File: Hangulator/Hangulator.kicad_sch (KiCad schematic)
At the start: 78 parts, among them J1 Conn_01x02_Male, J2 Conn_01x02_Male, U1 AMS1117-3.3, U2 STM32F072VBTx

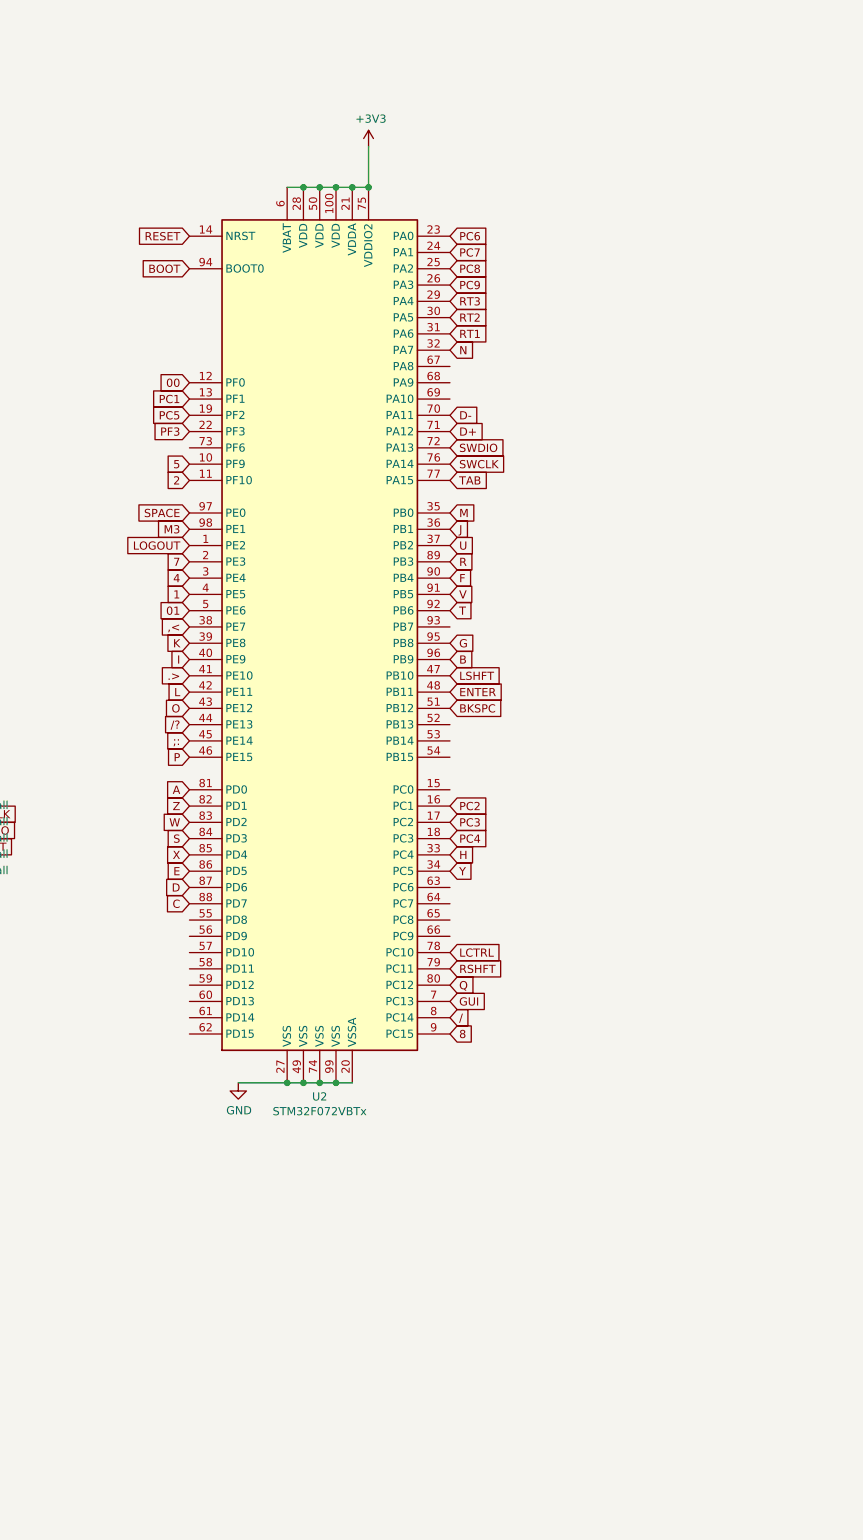
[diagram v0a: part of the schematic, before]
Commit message: lol
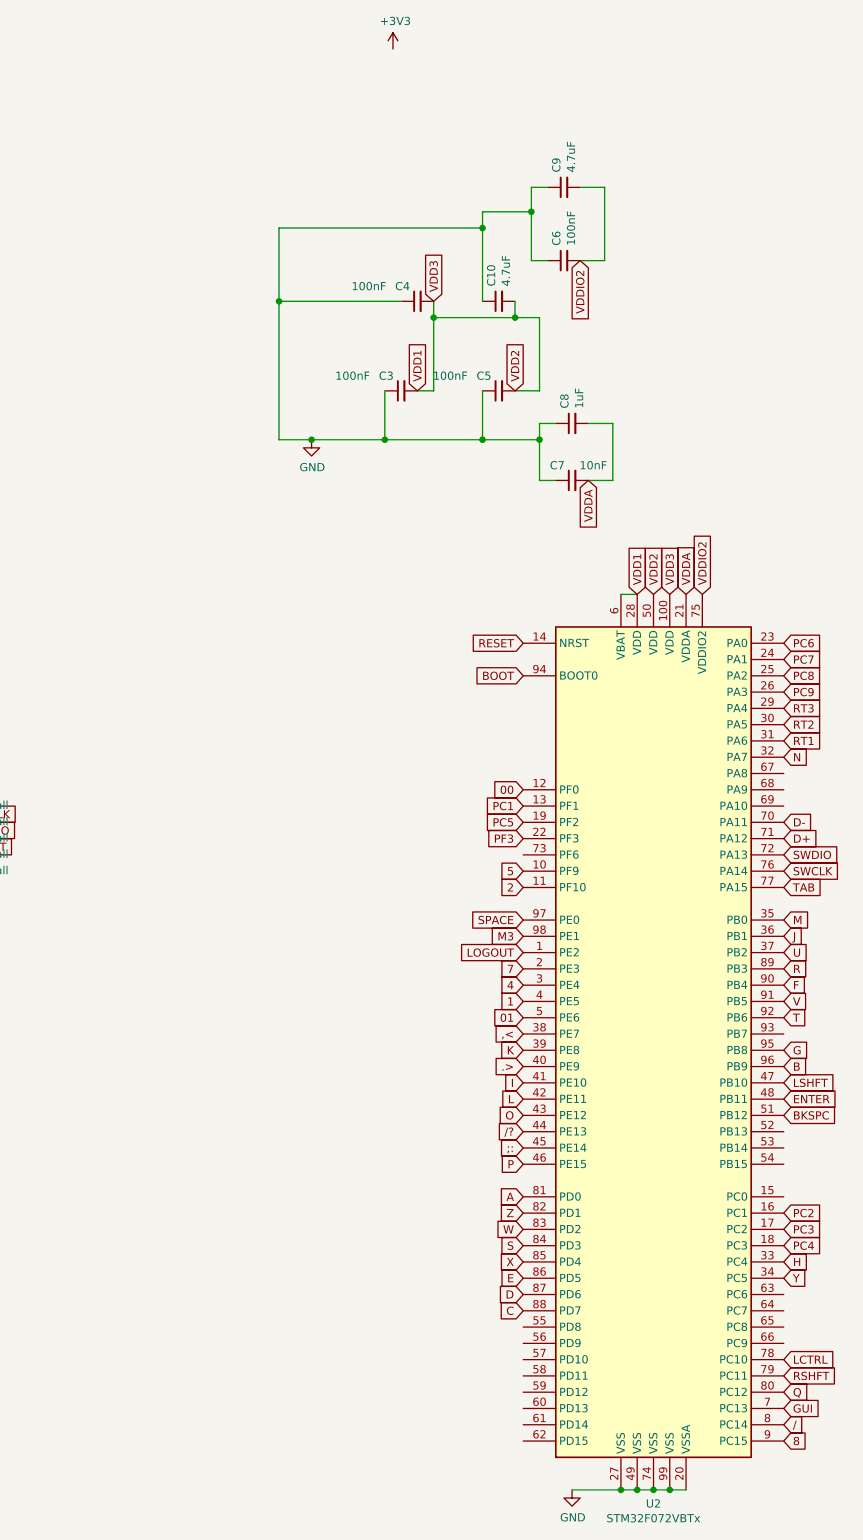
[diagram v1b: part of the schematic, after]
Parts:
- added C10, C9: 4.7uF, Capacitor_SMD:C_0603_1608Metric_Pad1.08x0.95mm_HandSolder, symbol Device:C_Small
- added C3, C4, C5, C6: 100nF, Capacitor_SMD:C_0805_2012Metric_Pad1.18x1.45mm_HandSolder, symbol Device:C_Small
- added C7: 10nF, Capacitor_SMD:C_0805_2012Metric_Pad1.18x1.45mm_HandSolder, symbol Device:C_Small
- added C8: 1uF, Capacitor_SMD:C_0805_2012Metric_Pad1.18x1.45mm_HandSolder, symbol Device:C_Small
- C1, C2: footprint Capacitor_SMD:C_0603_1608Metric_Pad1.08x0.95mm_HandSolder -> Capacitor_SMD:C_0805_2012Metric_Pad1.18x1.45mm_HandSolder
- R1, R2, R3, R4: footprint Resistor_SMD:R_0603_1608Metric_Pad0.98x0.95mm_HandSolder -> Resistor_SMD:R_0805_2012Metric_Pad1.20x1.40mm_HandSolder
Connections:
- net +3V3: no longer U2.100 (VDD), U2.21 (VDDA), U2.28 (VDD), U2.50 (VDD), U2.6 (VBAT), U2.75 (VDDIO2)
- net .>: now also U2.40 (PE9); no longer U2.41 (PE10)
- net GND: now also C10.1, C3.1, C4.1, C5.1, C6.1, C7.1, C8.1, C9.1
- net I: now also U2.41 (PE10); no longer U2.40 (PE9)
- new net VDD1: C10.2, C3.2, C4.2, C5.2, U2.100 (VDD), U2.28 (VDD), U2.50 (VDD), U2.6 (VBAT)
- new net VDDA: C7.2, C8.2, U2.21 (VDDA)
- new net VDDIO2: C6.2, C9.2, U2.75 (VDDIO2)
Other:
- moved on the sheet: U2
